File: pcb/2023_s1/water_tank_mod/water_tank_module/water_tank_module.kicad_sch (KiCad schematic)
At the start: 9 parts, among them J2 Conn_01x05_Male, U4 NRF24L01_Breakout

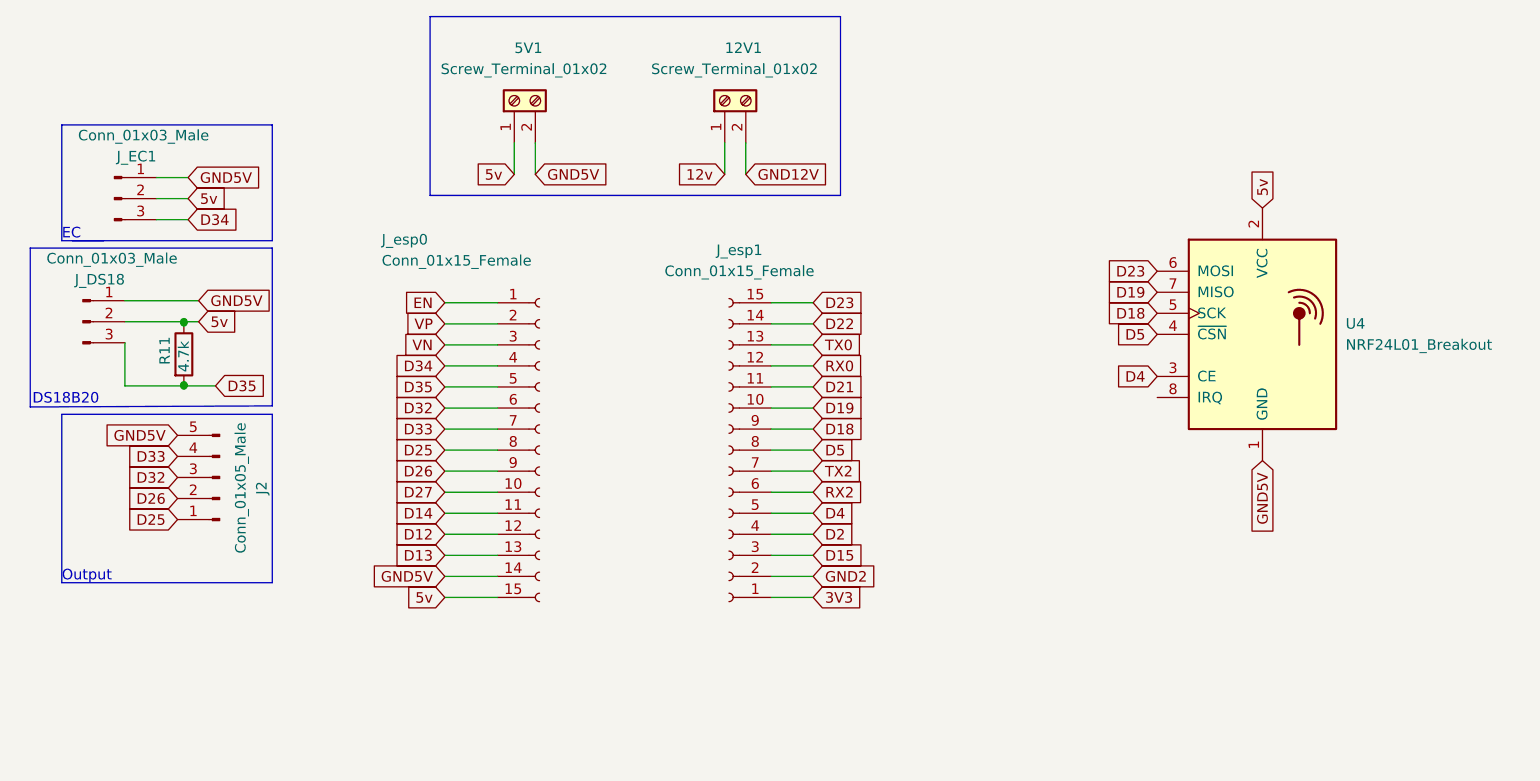
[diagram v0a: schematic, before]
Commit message: update, added 3d shapes for the pieces, and added capacitor
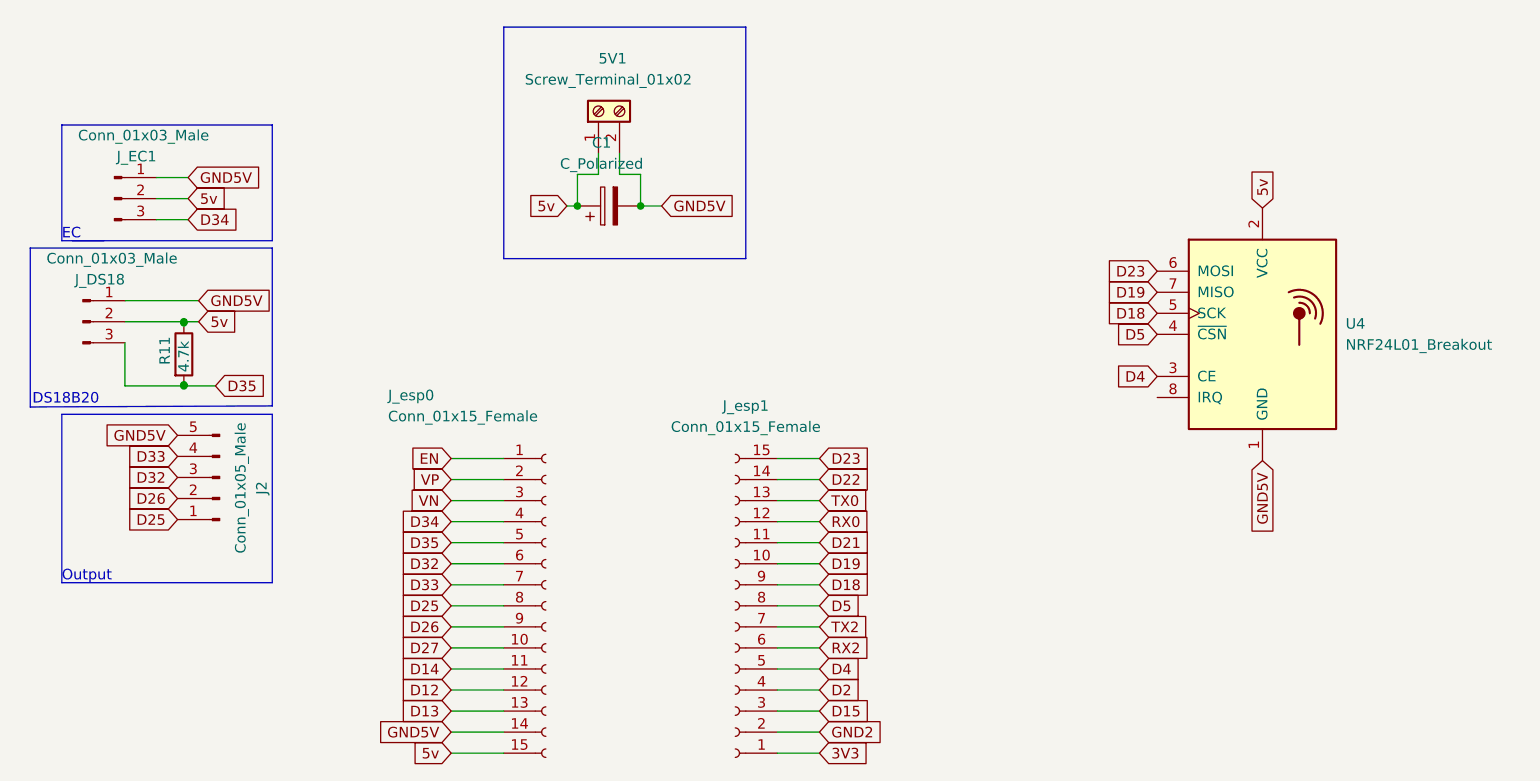
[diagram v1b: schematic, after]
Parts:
- removed 12V1: Screw_Terminal_01x02, TerminalBlock:TerminalBlock_Altech_AK300-2_P5.00mm, symbol Connector:Screw_Terminal_01x02
- added C1: C_Polarized, symbol Device:C_Polarized
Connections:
- net 5v: now also C1.1
- net GND5V: now also C1.2
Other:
- moved on the sheet: 5V1, J_esp0, J_esp1
